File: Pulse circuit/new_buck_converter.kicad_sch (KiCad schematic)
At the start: 7 parts, among them U5 MP1584EN(SOIC8E)

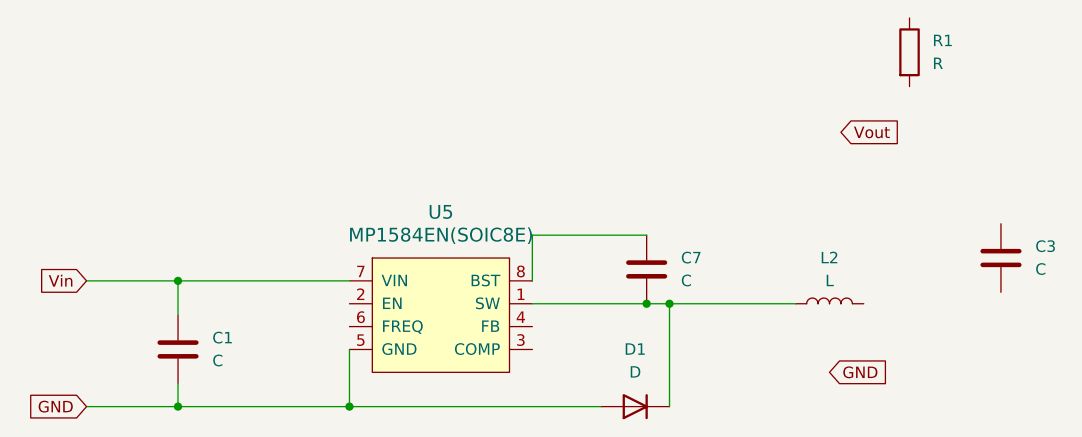
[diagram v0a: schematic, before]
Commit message: Changed the annotations
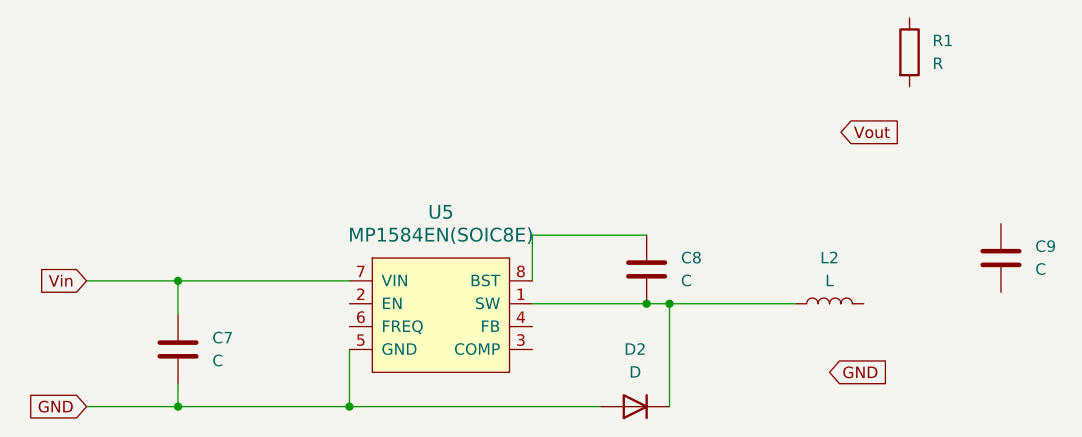
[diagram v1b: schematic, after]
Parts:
- renumbered C1 to C7, C7 to C8, C3 to C9, D1 to D2
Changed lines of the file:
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@@
 		(dnp no)
 		(fields_autoplaced yes)
-		(property "Reference" "D1"
+		(property "Reference" "D2"
 			(at 158.75 95.25 0)
 			(effects
@@
 			(project "Pulse circuit"
 				(path "/59caed24-c499-43df-90b9-3ac3a8609322/0afa37a8-64ca-4e6b-9013-61cb70edd3e2"
-					(reference "D1")
+					(reference "D2")
 					(unit 1)
 				)
@@
 		(dnp no)
 		(fields_autoplaced yes)
-		(property "Reference" "C3"
+		(property "Reference" "C9"
 			(at 203.2 83.8199 0)
 			(effects
@@
 			(project ""
 				(path "/59caed24-c499-43df-90b9-3ac3a8609322/0afa37a8-64ca-4e6b-9013-61cb70edd3e2"
-					(reference "C3")
+					(reference "C9")
 					(unit 1)
 				)
@@
 		(dnp no)
 		(fields_autoplaced yes)
-		(property "Reference" "C1"
+		(property "Reference" "C7"
 			(at 111.76 93.9799 0)
 			(effects
@@
 			(project "Pulse circuit"
 				(path "/59caed24-c499-43df-90b9-3ac3a8609322/0afa37a8-64ca-4e6b-9013-61cb70edd3e2"
-					(reference "C1")
+					(reference "C7")
 					(unit 1)
 				)
@@
 		(dnp no)
 		(fields_autoplaced yes)
-		(property "Reference" "C7"
+		(property "Reference" "C8"
 			(at 163.83 85.0899 0)
 			(effects
@@
 			(project ""
 				(path "/59caed24-c499-43df-90b9-3ac3a8609322/0afa37a8-64ca-4e6b-9013-61cb70edd3e2"
-					(reference "C7")
-					(unit 1)
-				)
+					(reference "C8")
+					(unit 1)
+				)

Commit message: values added to buck converter
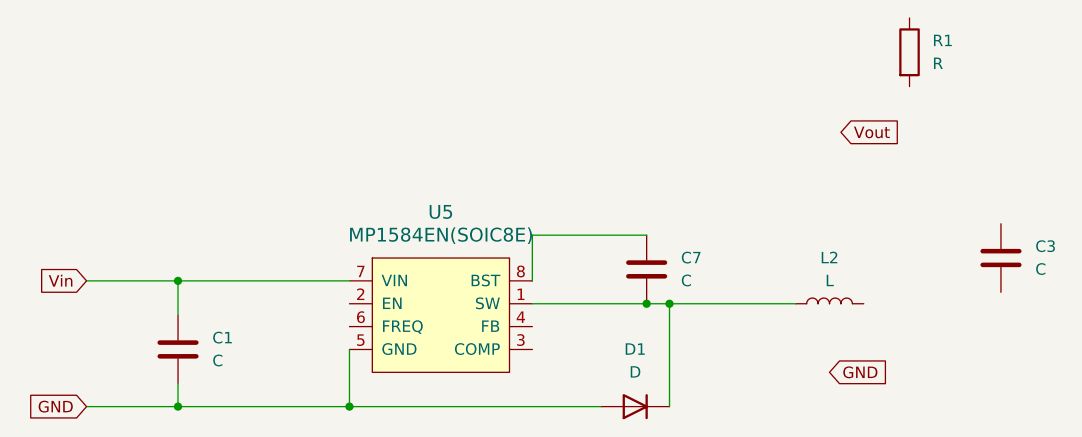
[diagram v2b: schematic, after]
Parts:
- renumbered C7 to C1, C9 to C3, C8 to C7, D2 to D1
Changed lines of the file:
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@@
 		(dnp no)
 		(fields_autoplaced yes)
-		(property "Reference" "D2"
+		(property "Reference" "D1"
 			(at 158.75 95.25 0)
 			(effects
@@
 			(project "Pulse circuit"
 				(path "/59caed24-c499-43df-90b9-3ac3a8609322/0afa37a8-64ca-4e6b-9013-61cb70edd3e2"
-					(reference "D2")
+					(reference "D1")
 					(unit 1)
 				)
@@
 		(dnp no)
 		(fields_autoplaced yes)
-		(property "Reference" "C9"
+		(property "Reference" "C3"
 			(at 203.2 83.8199 0)
 			(effects
@@
 			(project ""
 				(path "/59caed24-c499-43df-90b9-3ac3a8609322/0afa37a8-64ca-4e6b-9013-61cb70edd3e2"
-					(reference "C9")
+					(reference "C3")
 					(unit 1)
 				)
@@
 		(dnp no)
 		(fields_autoplaced yes)
-		(property "Reference" "C7"
+		(property "Reference" "C1"
 			(at 111.76 93.9799 0)
 			(effects
@@
 			(project "Pulse circuit"
 				(path "/59caed24-c499-43df-90b9-3ac3a8609322/0afa37a8-64ca-4e6b-9013-61cb70edd3e2"
-					(reference "C7")
+					(reference "C1")
 					(unit 1)
 				)
@@
 		(dnp no)
 		(fields_autoplaced yes)
-		(property "Reference" "C8"
+		(property "Reference" "C7"
 			(at 163.83 85.0899 0)
 			(effects
@@
 			(project ""
 				(path "/59caed24-c499-43df-90b9-3ac3a8609322/0afa37a8-64ca-4e6b-9013-61cb70edd3e2"
-					(reference "C8")
-					(unit 1)
-				)
+					(reference "C7")
+					(unit 1)
+				)
